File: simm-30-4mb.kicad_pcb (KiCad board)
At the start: 4 copper layers, 88.9 x 19 mm, 8 parts, among them J1 DRAM-SIMM-30, U1 AS4C4M4, U2 AS4C4M4

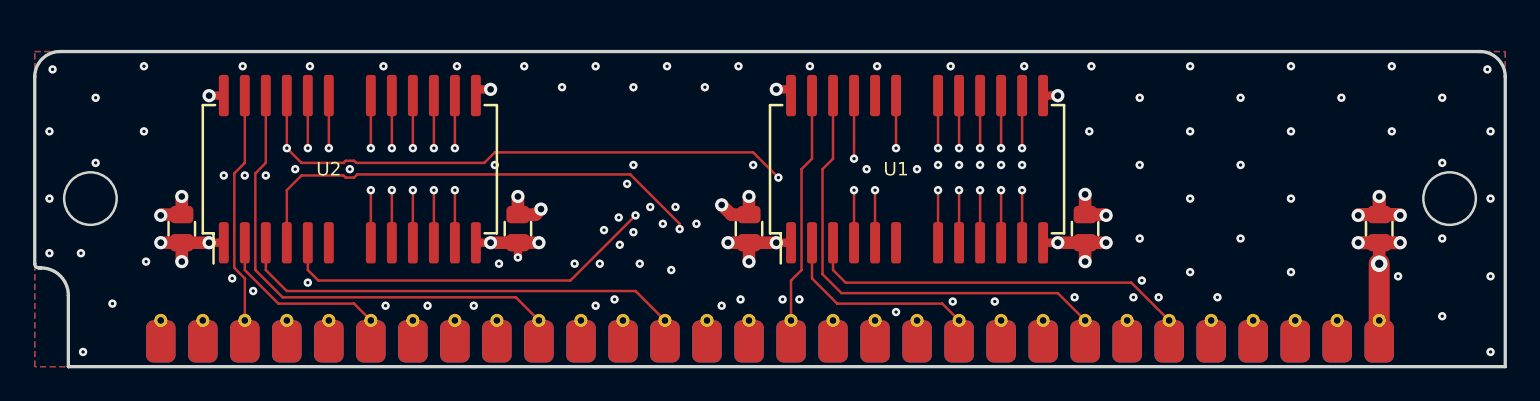
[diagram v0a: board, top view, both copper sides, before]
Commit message: Taller (20mm height)
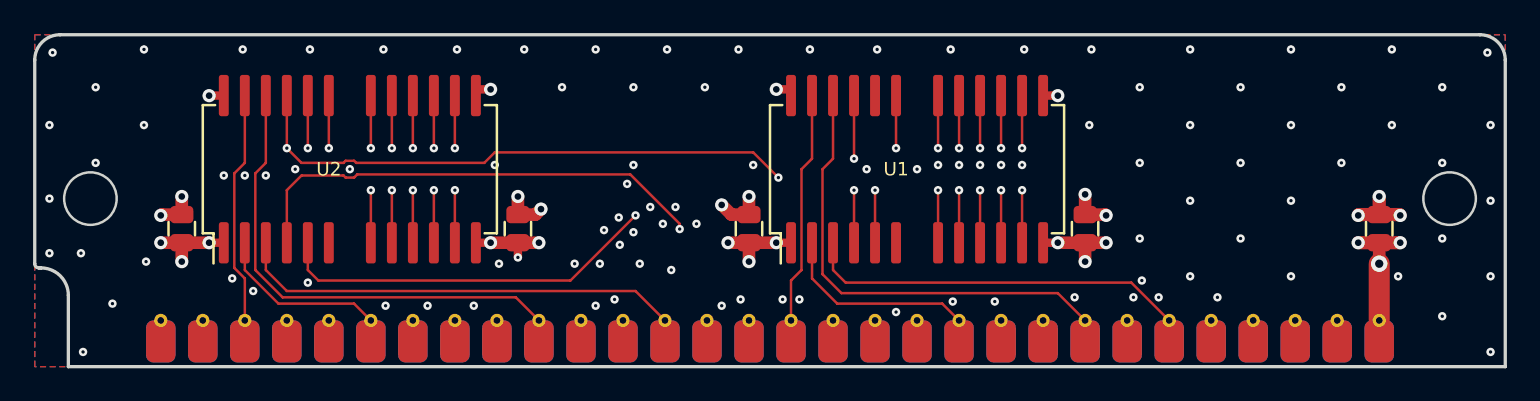
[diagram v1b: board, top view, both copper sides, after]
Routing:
- net GND: vias 121 -> 122
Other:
- board size 88.9 x 19 mm -> 88.9 x 20.1 mm
